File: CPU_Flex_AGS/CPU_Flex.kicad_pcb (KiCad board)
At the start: 2 copper layers, 20.5 x 21.3 mm, 4 parts, among them J3 Conn_01x16, J4 CPU_AGB_B_Interface

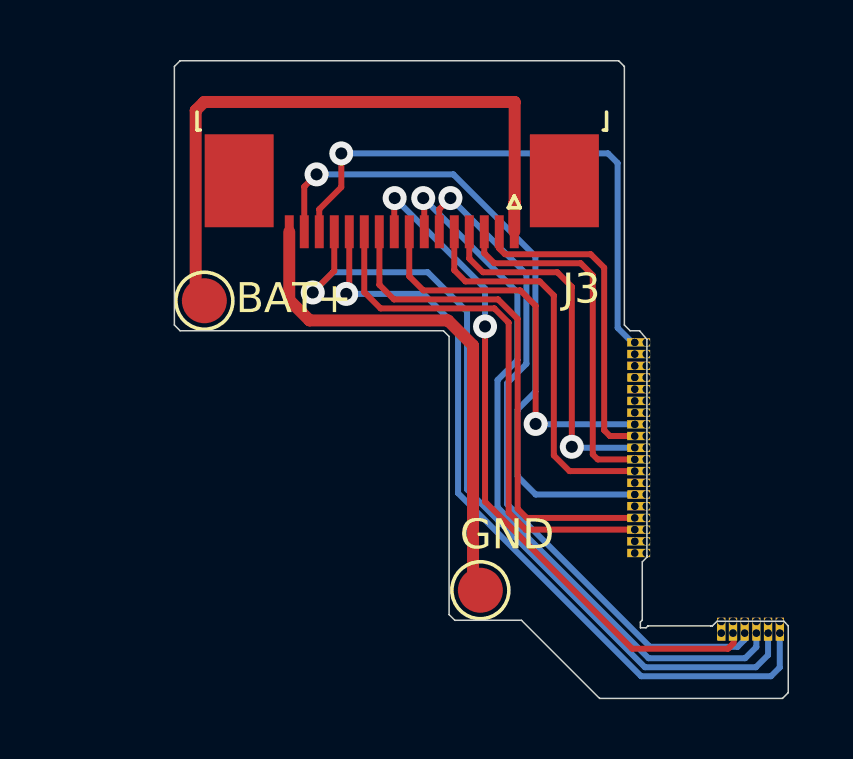
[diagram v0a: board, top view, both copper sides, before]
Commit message: updated CPU-flex
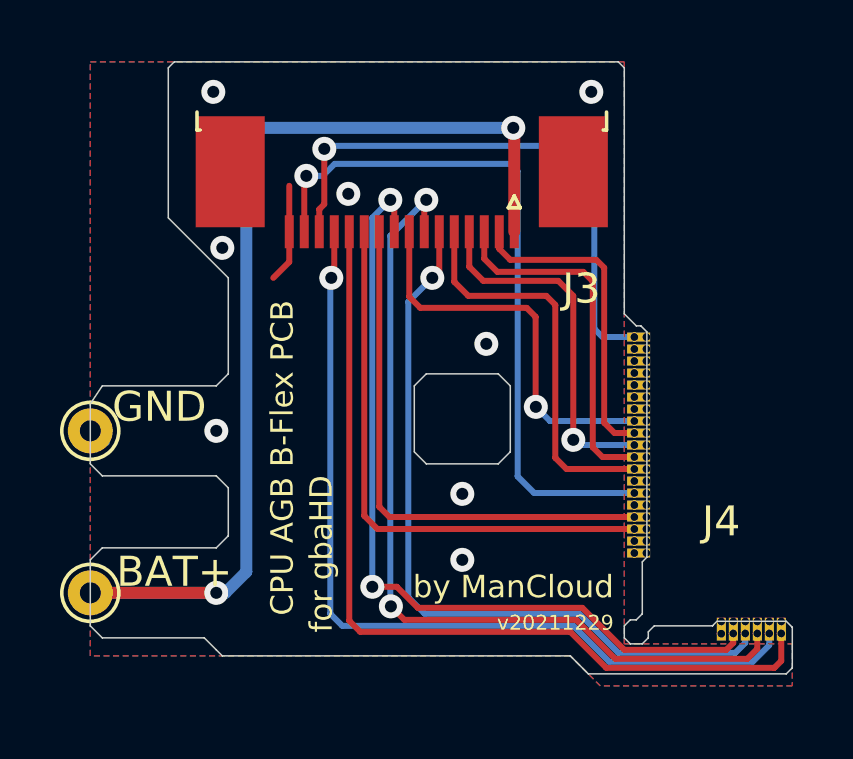
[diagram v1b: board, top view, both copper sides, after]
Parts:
- BAT+, GND: footprint TestPoint:TestPoint_Pad_D1.5mm -> TestPoint:TestPoint_THTPad_D1.5mm_Drill0.7mm
- J4: footprint Nintendo:CPU_AGB_B_Interface -> Ninteno:CPU_AGB_B_Interface
- moved GND 14.0 mm to (94.7, 87.3)
- moved BAT+ 10.5 mm to (94.7, 92.7)
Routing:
- net VCC: track 21.5 -> 36.1 mm, vias 0 -> 2
- net GND: track 17.3 -> 5.40 mm, vias 0 -> 8
- net /GBA_R: track 23.1 -> 27.6 mm
- net /GBA_B: track 24.5 -> 28.7 mm, vias 1 -> 2
- net /GBA_AUD_L: track 26.5 -> 29.0 mm, vias 1 -> 0
- net /GBA_A: track 23.2 -> 25.1 mm
- net /GBA_RESET: track 22.4 -> 23.5 mm
- net /GBA_AUD_R: track 27.8 -> 28.7 mm
- added copper zone on B.Cu, net GND
- added copper zone on F.Cu, net GND
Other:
- board size 20.5 x 21.3 mm -> 23.4 x 20.4 mm
- net class Default removed
- board text added: "CPU AGB B-Flex PCB"
- board text added: "by ManCloud"
- board text added: "for gbaHD"
- board text added: "v20211229"
